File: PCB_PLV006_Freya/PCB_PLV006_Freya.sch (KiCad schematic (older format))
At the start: 32 parts

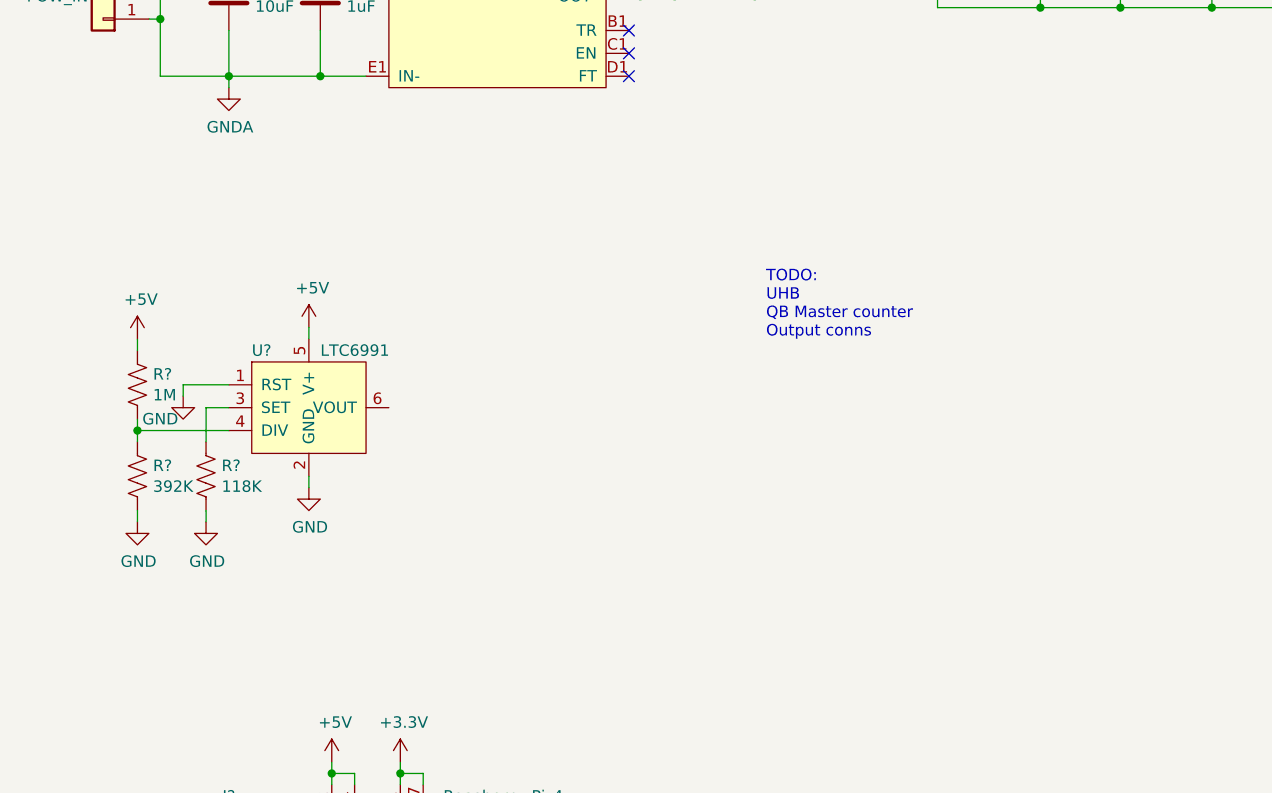
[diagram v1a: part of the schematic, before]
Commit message: Freya stuff
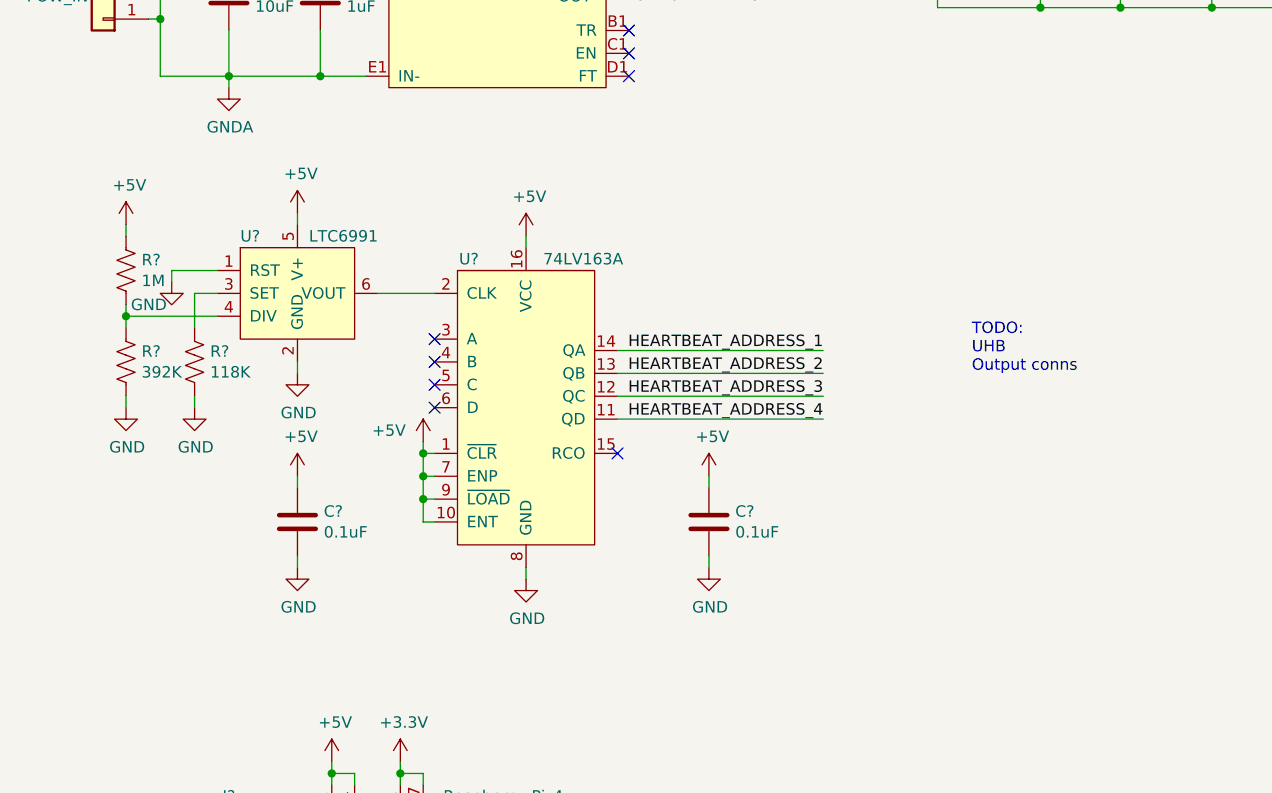
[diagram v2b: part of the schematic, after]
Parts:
- added C? (x2): 0.1uF, symbol Device:C
- added U?: 74LV163A, symbol boringlib:74LV163A
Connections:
- net +5V: now also C?.1, C?.1, U?.1 (~CLR~), U?.10 (ENT), U?.16 (VCC), U?.7 (ENP), U?.9 (~LOAD~)
- net GND: now also C?.2, C?.2, U?.8 (GND)
- net at U?.6 (VOUT): now also U?.2 (CLK)
- new net HEARTBEAT_ADDRESS_1: U?.14 (QA)
- new net HEARTBEAT_ADDRESS_2: U?.13 (QB)
- new net HEARTBEAT_ADDRESS_3: U?.12 (QC)
- new net HEARTBEAT_ADDRESS_4: U?.11 (QD)
- no-connect marks 14 -> 19
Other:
- note added: "TODO:\nUHB\nOutput conns\n"
- note removed: "TODO:\nUHB\nQB Master counter\nOutput conns\n"
- moved on the sheet: R?, U?
